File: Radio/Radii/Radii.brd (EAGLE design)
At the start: 43.1 x 44.3 mm, 14 parts, among them U2 74HC4050D,653

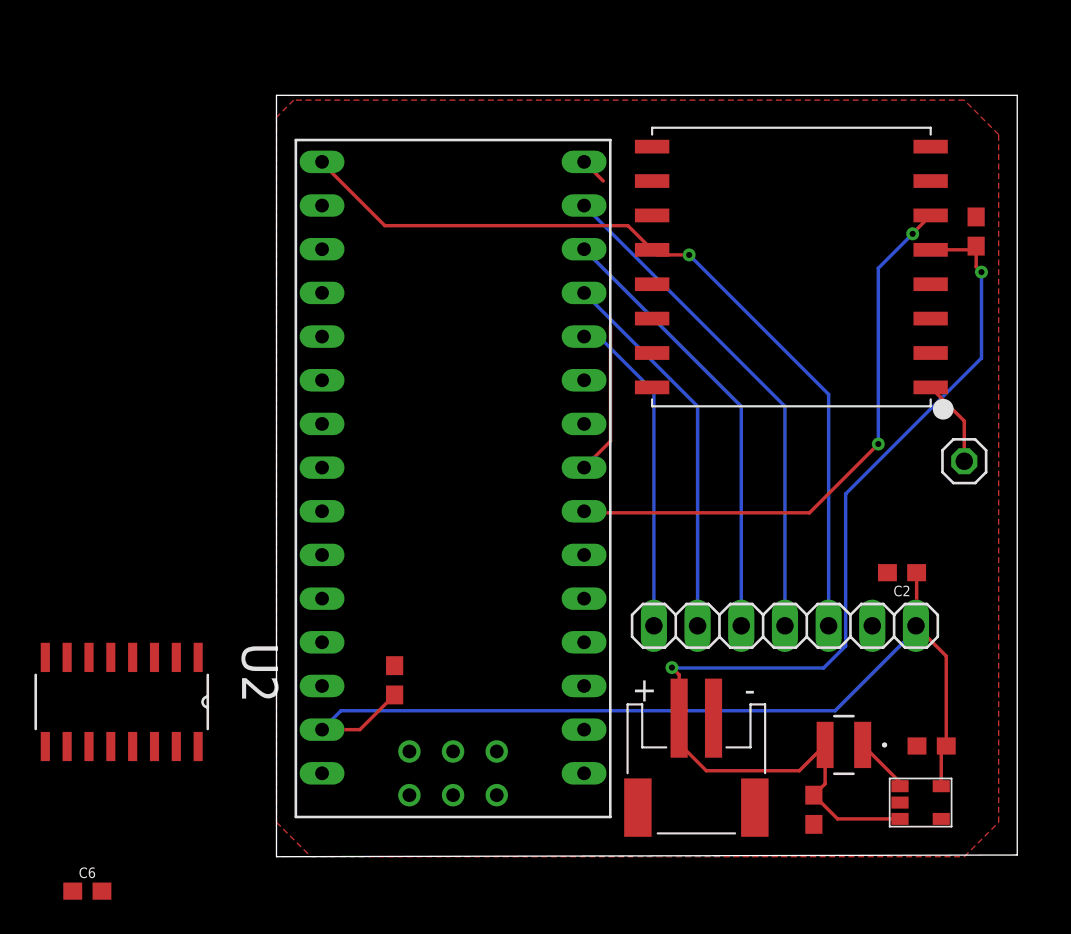
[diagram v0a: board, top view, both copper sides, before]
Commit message: Updated board with Level Shifter
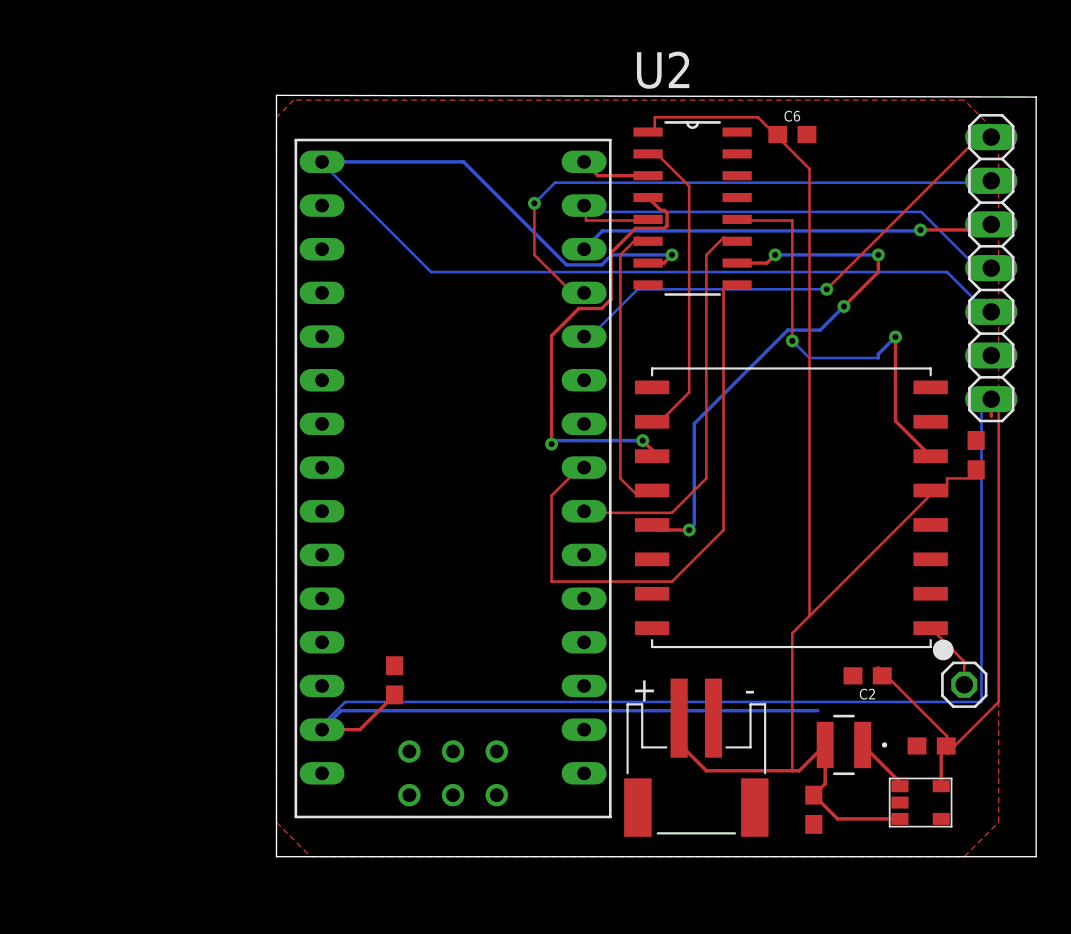
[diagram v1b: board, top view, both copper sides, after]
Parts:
- U2: value 74HC4050D,653 -> LEV_SHIFT
- moved C6 60.1 mm to (30.0, 42.0)
- moved U2 43.9 mm to (24.2, 37.7), turned to 0 degrees
- moved JP1 24.0 mm to (41.6, 34.2), turned to 90 degrees
- moved U1 14.0 mm to (29.9, 20.3)
- moved C3 13.0 mm to (40.7, 23.4)
- moved JP2 13.0 mm to (40.0, 10.0)
- moved C2 6.32 mm to (34.4, 10.5)
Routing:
- net 5V: track 55.5 -> 124.4 mm
- net SCK5: track 26.8 -> 67.2 mm
- net SS3: track 0.00 -> 32.3 mm, vias 0 -> 4
- net MOSI3: track 0.00 -> 26.0 mm, vias 0 -> 2
- net SS5: track 8.88 -> 33.6 mm
- net INT5: track 0.00 -> 23.2 mm
- net 3.3V: track 63.2 -> 82.0 mm, vias 2 -> 0
- net MISO3: track 0.00 -> 18.4 mm
- net DISP_RESET: track 22.1 -> 33.8 mm, vias 0 -> 1
- net DC_SELECT: track 17.8 -> 28.8 mm, vias 0 -> 1
- net INT: track 33.2 -> 25.1 mm
- net SCK3: track 20.8 -> 17.4 mm
- net MISO5: track 1.58 -> 4.05 mm
- net CS5: track 25.7 -> 24.3 mm, vias 0 -> 1
- net N$3: track 5.10 -> 4.10 mm
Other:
- board size 43.1 x 44.3 mm -> 44.2 x 44.3 mm
